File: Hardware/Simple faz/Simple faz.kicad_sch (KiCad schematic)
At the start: 45 parts, among them J1 Entrada, J2 Re1, J3 Re1, J4 Re1, J5 Re1, K1 PR14-12V-360-1C, K2 PR14-12V-360-1C, K3 PR14-12V-360-1C, K4 PR14-12V-360-1C, Q1 MMBT2222A, Q2 MMBT2222A, Q3 MMBT2222A, Q4 MMBT2222A, U1 PC817, U2 PC817, U3 PC817, U4 PC817, U5 DEVKIT_V1_ESP32-WROOM-32

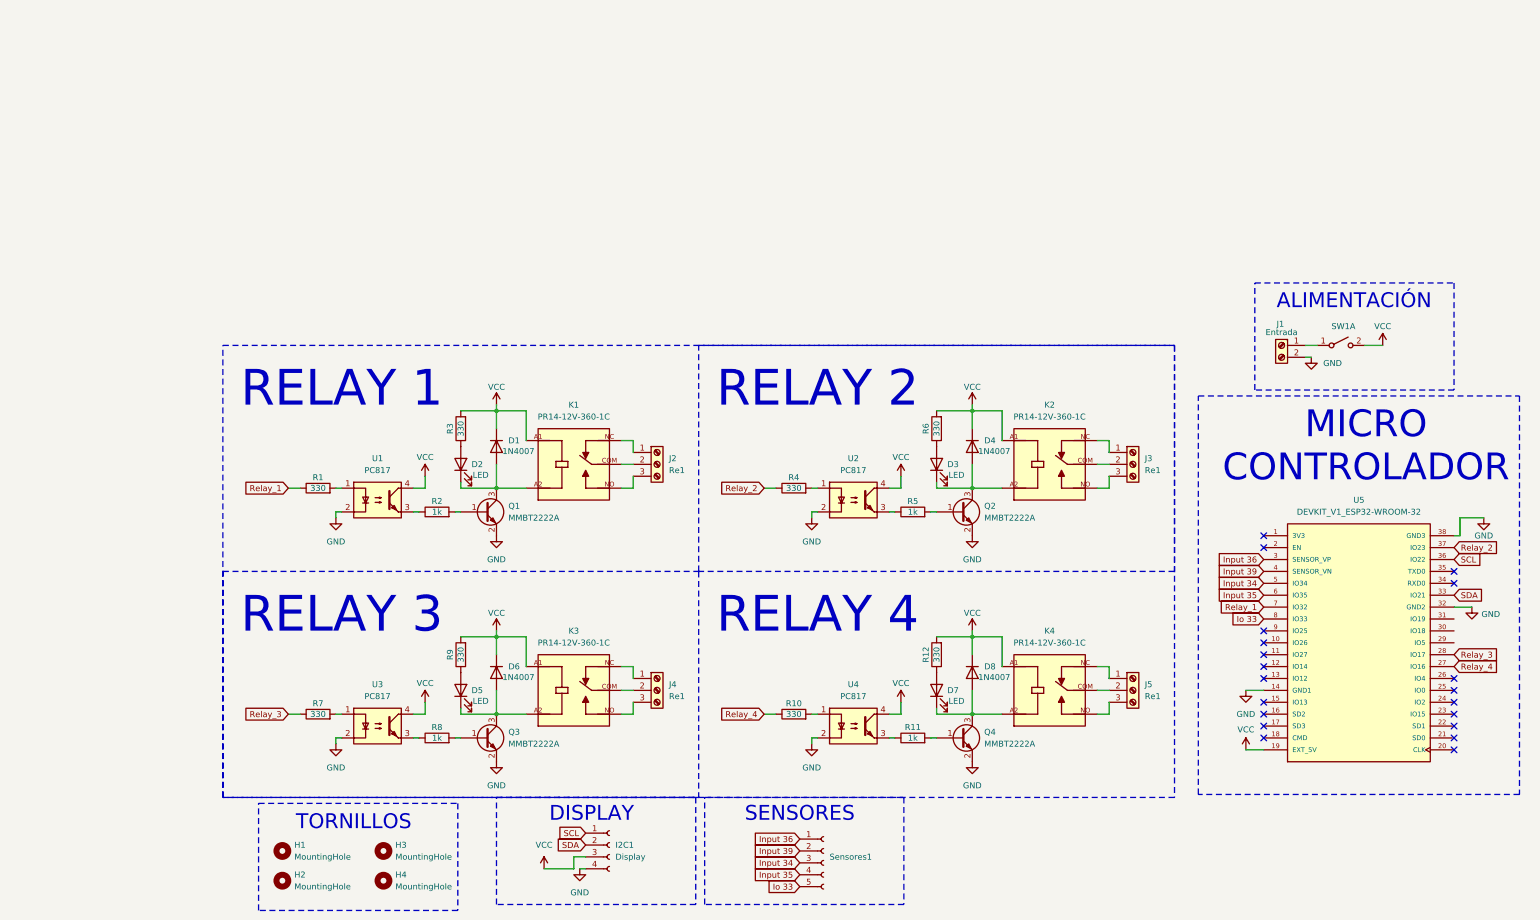
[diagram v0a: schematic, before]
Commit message: Ultima version
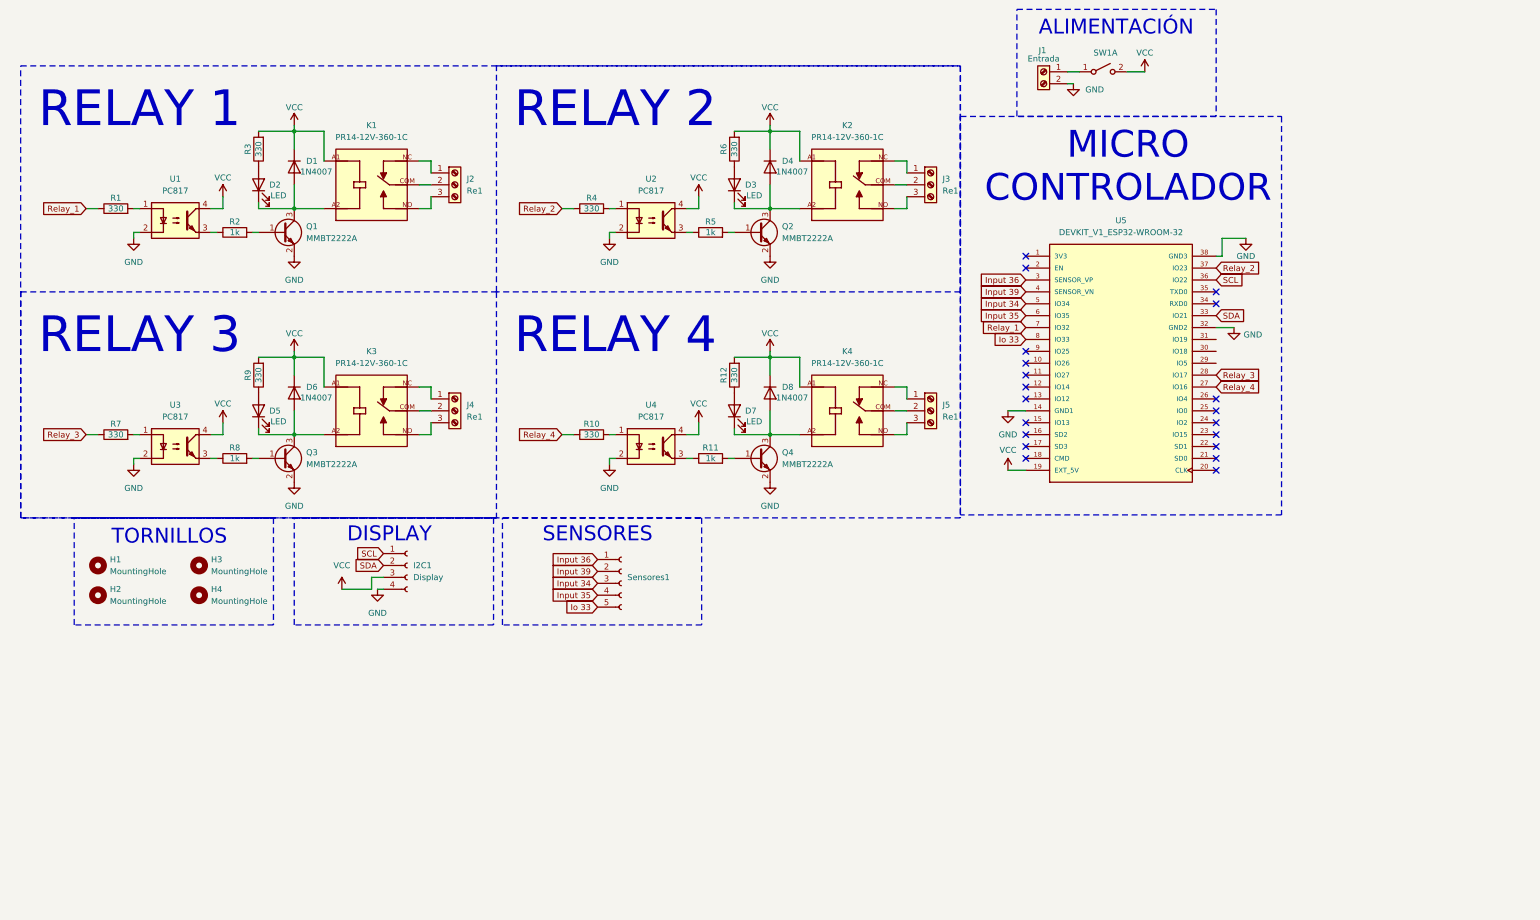
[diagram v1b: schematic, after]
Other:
- moved on the sheet: D1, D2, D3, D4, D5, D6, D7, D8, H1, H2, H3, H4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
